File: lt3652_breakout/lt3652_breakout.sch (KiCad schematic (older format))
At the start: 24 parts, among them CON1 SLR PNL, U1 LT3652

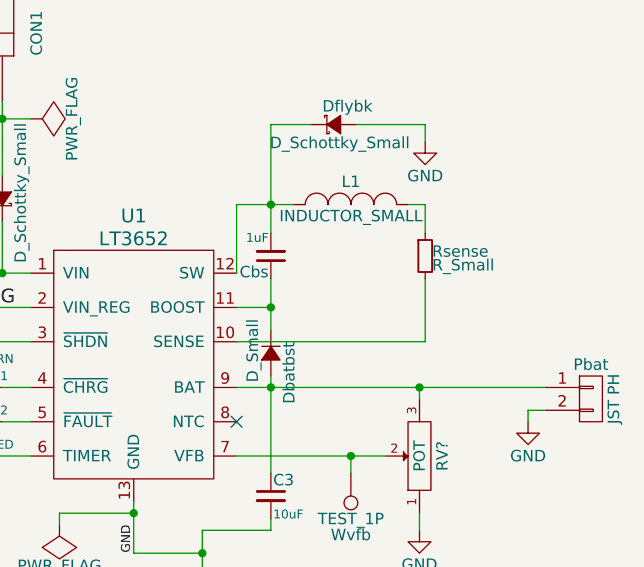
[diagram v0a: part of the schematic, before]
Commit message: WIP on Rev 0.2
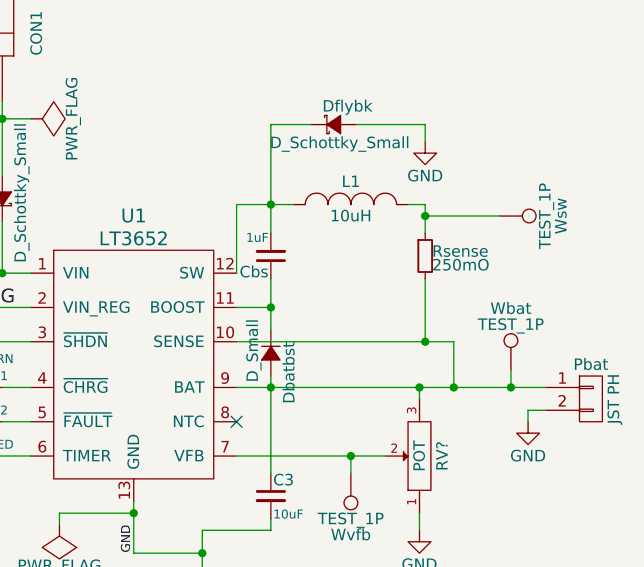
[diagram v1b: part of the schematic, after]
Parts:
- added Wbat, Wsw: TEST_1P, pcb_test_points:KEYSTONE_5016_PCB_Test_Point, symbol TEST_1P
- L1: value INDUCTOR_SMALL -> 10uH
- Rsense: value R_Small -> 250mO
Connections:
- net at Rsense.2, U1.10 (SENSE): now also C3.1, Dbatbst.2 (A), Pbat.1 (P1), RV?.3, U1.9 (BAT), Wbat.1
- net at L1.2, Rsense.1: now also Wsw.1
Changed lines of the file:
@@
 P 6450 2750
 F 0 "L1" H 6450 2850 50  0000 C CNN
-F 1 "INDUCTOR_SMALL" H 6450 2700 50  0000 C CNN
+F 1 "10uH" H 6450 2700 50  0000 C CNN
 F 2 "" H 6450 2750 50  0000 C CNN
 F 3 "" H 6450 2750 50  0000 C CNN
@@
 P 6775 2975
 F 0 "Rsense" H 6805 2995 50  0000 L CNN
-F 1 "R_Small" H 6805 2935 50  0000 L CNN
+F 1 "250mO" H 6805 2935 50  0000 L CNN
 F 2 "" H 6775 2975 50  0000 C CNN
 F 3 "" H 6775 2975 50  0000 C CNN
@@
 Connection ~ 6100 3550
 Wire Wire Line
-	5950 3350 6775 3350
+	5950 3350 6900 3350
 Wire Wire Line
 	6775 3350 6775 3075
@@
 Wire Wire Line
 	4925 2825 4925 3050
+Wire Wire Line
+	6900 3350 6900 3550
+Connection ~ 6900 3550
+Connection ~ 6775 3350
+$Comp
+L TEST_1P Wbat
+U 1 1 56CEBC53
+P 7150 3475
+F 0 "Wbat" H 7150 3745 50  0000 C CNN
+F 1 "TEST_1P" H 7150 3675 50  0000 C CNN
+F 2 "pcb_test_points:KEYSTONE_5016_PCB_Test_Point" H 7350 3475 50  0001 C CNN
+F 3 "" H 7350 3475 50  0000 C CNN
+	1    7150 3475
+	1    0    0    -1
+$EndComp
+Wire Wire Line
+	7150 3475 7150 3550
+Connection ~ 7150 3550
+$Comp
+L TEST_1P Wsw
+U 1 1 56CEC1FA
+P 7100 2800
+F 0 "Wsw" H 7100 3070 50  0000 C CNN
+F 1 "TEST_1P" H 7100 3000 50  0000 C CNN
+F 2 "pcb_test_points:KEYSTONE_5016_PCB_Test_Point" H 7300 2800 50  0001 C CNN
+F 3 "" H 7300 2800 50  0000 C CNN
+	1    7100 2800
+	0    1    1    0
+$EndComp
+Wire Wire Line
+	7100 2800 6775 2800
+Connection ~ 6775 2800
 $EndSCHEMATC
